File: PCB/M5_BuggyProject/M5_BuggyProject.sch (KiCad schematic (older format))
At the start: 25 parts, among them J1 XT60, J2 VCC, J3 10V, J4 Receiver

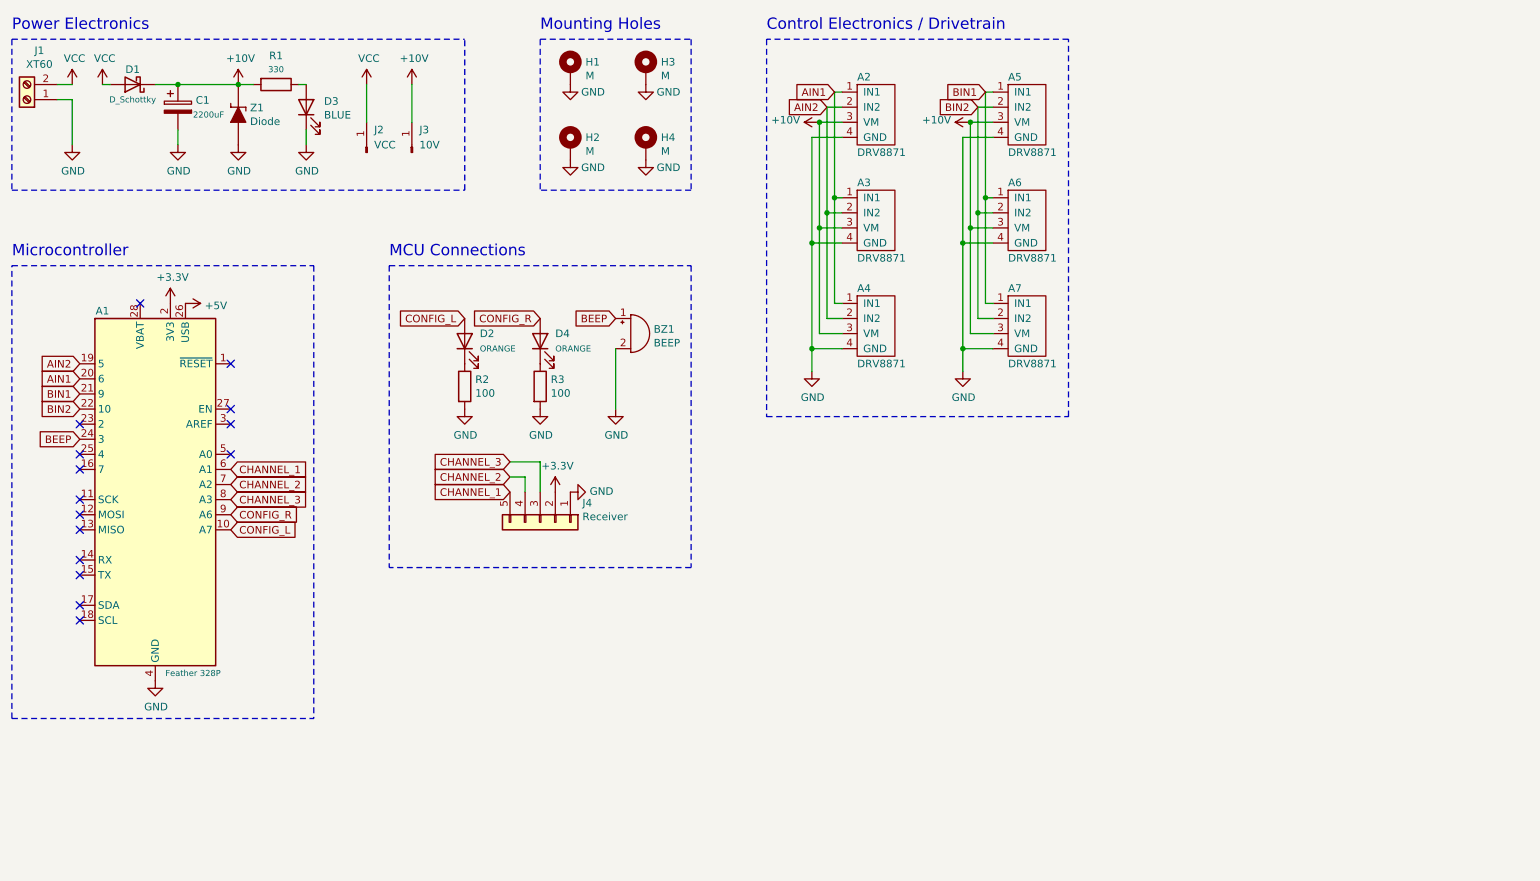
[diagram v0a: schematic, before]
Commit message: Started PCB v2
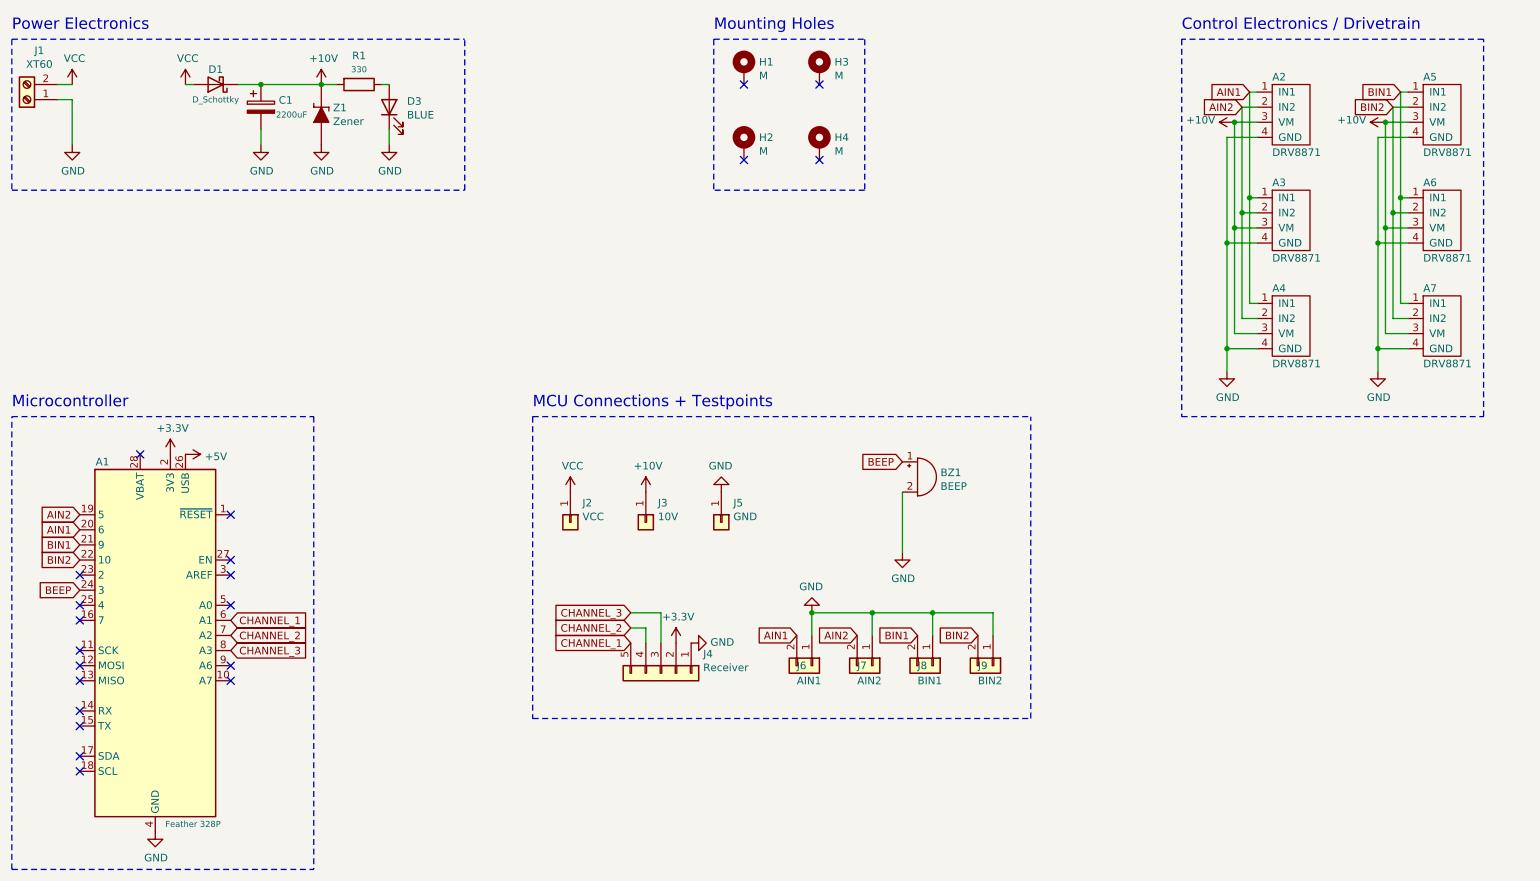
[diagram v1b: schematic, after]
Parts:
- removed D2, D4: ORANGE, LED_SMD:LED_1206_3216Metric, symbol Device:LED
- removed J2: VCC, TestPoint:TestPoint_Loop_D1.80mm_Drill1.0mm_Beaded, symbol Connector:Conn_01x01_Male
- removed J3: 10V, TestPoint:TestPoint_Loop_D1.80mm_Drill1.0mm_Beaded, symbol Connector:Conn_01x01_Male
- removed R2, R3: 100, Resistor_SMD:R_1206_3216Metric, symbol Device:R
- added J2: VCC, TestPoint:TestPoint_Plated_Hole_D5.0mm, symbol Connector_Generic:Conn_01x01
- added J3: 10V, TestPoint:TestPoint_Plated_Hole_D5.0mm, symbol Connector_Generic:Conn_01x01
- added J5: GND, TestPoint:TestPoint_Plated_Hole_D5.0mm, symbol Connector_Generic:Conn_01x01
- added J6: AIN1, Connector_PinSocket_2.54mm:PinSocket_1x02_P2.54mm_Vertical, symbol Connector_Generic:Conn_01x02
- added J7: AIN2, Connector_PinSocket_2.54mm:PinSocket_1x02_P2.54mm_Vertical, symbol Connector_Generic:Conn_01x02
- added J8: BIN1, Connector_PinSocket_2.54mm:PinSocket_1x02_P2.54mm_Vertical, symbol Connector_Generic:Conn_01x02
- added J9: BIN2, Connector_PinSocket_2.54mm:PinSocket_1x02_P2.54mm_Vertical, symbol Connector_Generic:Conn_01x02
- H1, H2, H3, H4: footprint MountingHole:MountingHole_3.2mm_M3_Pad_Via -> MountingHole:MountingHole_4.3mm_M4_Pad_Via
- Z1: value Diode -> Zener
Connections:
- net +10V: now also J3.1 (Pin_1)
- net AIN1: now also J6.2 (Pin_2)
- net AIN2: now also J7.2 (Pin_2)
- net BIN1: now also J8.2 (Pin_2)
- net BIN2: now also J9.2 (Pin_2)
- net GND: now also J5.1 (Pin_1), J6.1 (Pin_1), J7.1 (Pin_1), J8.1 (Pin_1), J9.1 (Pin_1); no longer H1.1, H2.1, H3.1, H4.1
- net VCC: now also J2.1 (Pin_1)
- net CONFIG_L: no longer names the net of A1.10 (A7)
- net CONFIG_R: no longer names the net of A1.9 (A6)
- no-connect marks 15 -> 21
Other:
- note added: "MCU Connections + Testpoints"
- note removed: "MCU Connections"
- moved on the sheet: A1, A2, A3, A4, A5, A6, A7, BZ1, C1, D1, D3, H1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
